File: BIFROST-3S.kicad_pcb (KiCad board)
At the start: 2 copper layers, 60 x 40 mm, 8 parts, among them J2 200241-1222, J3 200241-1222, J4 B6B-XH-A_LF__SN_, J5 B4B-XH-A_LF__SN_, J6 560020-1020, J7 200241-1222

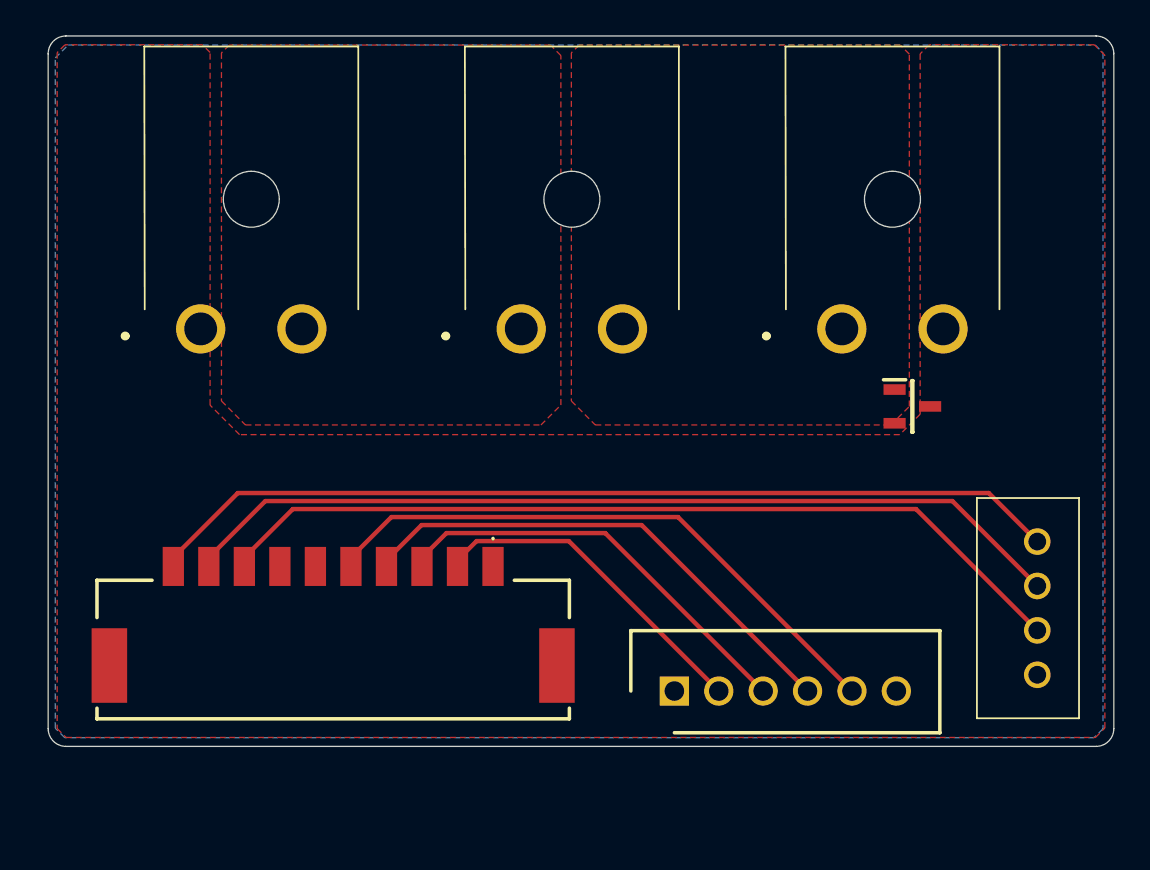
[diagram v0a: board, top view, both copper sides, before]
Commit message: Schematic+Layout 3.0
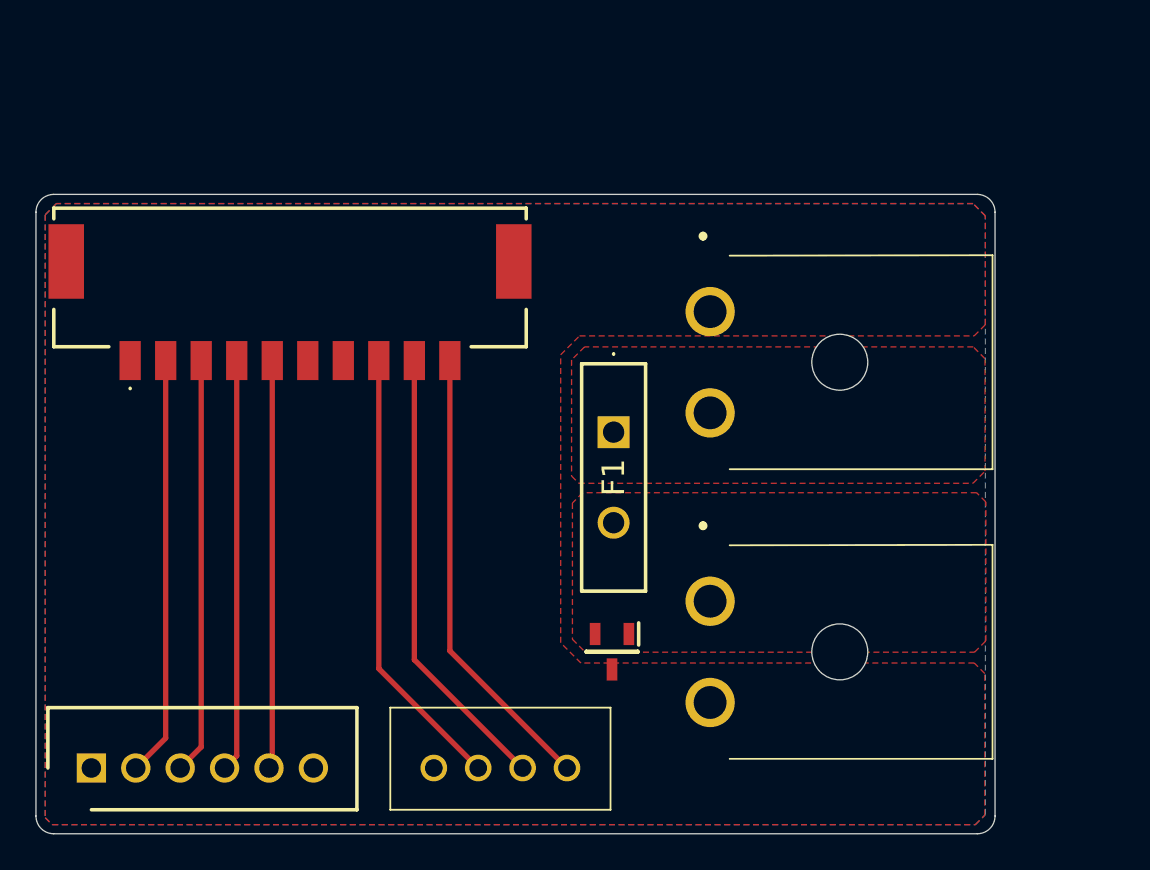
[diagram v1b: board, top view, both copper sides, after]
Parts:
- removed J2: 200241-1222, 200241-1222:2002411222
- added F1: MF-RHS800-0, MF-RHS800-0:MFRHS8000, F.Cu at (147.2, 100.1)
- moved J5 34.4 mm to (137.1, 119.0), turned to 0 degrees
- moved J4 33.1 mm to (117.8, 119.0)
- moved J7 28.7 mm to (152.6, 93.3), turned to 90 degrees
- moved D1 21.8 mm to (147.1, 112.4), turned to -90 degrees
- moved J6 21.1 mm to (129.0, 91.4), turned to 180 degrees
- moved J3 17.0 mm to (152.6, 109.6), turned to 90 degrees
- moved G*** 7.90 mm to (141.7, 104.7)
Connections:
- net /BAT3 renamed /BAT3/PACK+
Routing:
- net /BQ2_TS1: track 51.8 -> 25.7 mm
- net /BQ2_TS2: track 50.4 -> 25.5 mm
- net /BQ2_TS3: track 49.1 -> 25.3 mm
- net /BQ_TS: track 33.7 -> 23.0 mm
- net /BAT3/PACK+: track 28.8 -> 23.2 mm
- net /BAT1: track 19.0 -> 23.6 mm
- net /BAT2: track 24.0 -> 23.4 mm
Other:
- board size 60 x 40 mm -> 54 x 36 mm
